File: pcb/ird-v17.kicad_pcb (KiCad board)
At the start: 2 copper layers, 25.4 x 30.5 mm, 21 parts, among them J1 AVR-TPI-6, J2 Conn_02x06_Odd_Even, K1 G6K-2, Q1 NPN 10K, U1 ATtiny20-U, U2 TSOP75438WTT, U3 TLVM365R15RDNR

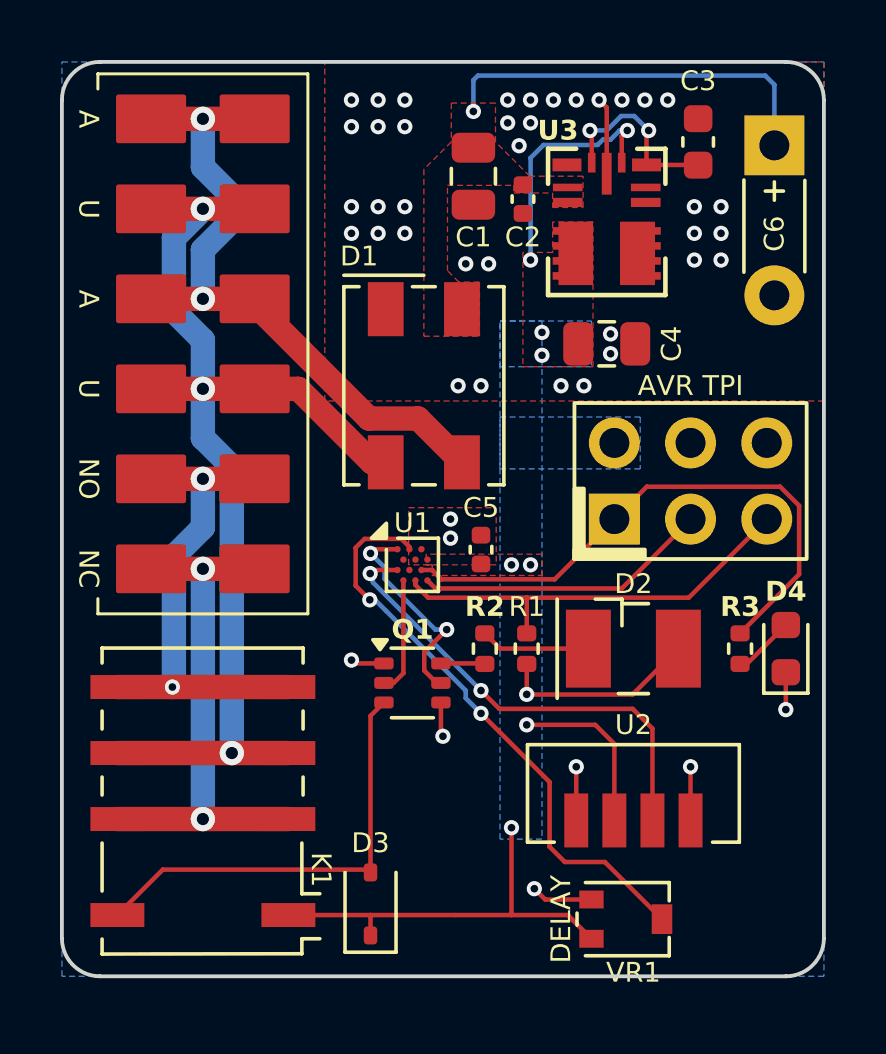
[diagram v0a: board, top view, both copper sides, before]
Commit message: Rearrange pins
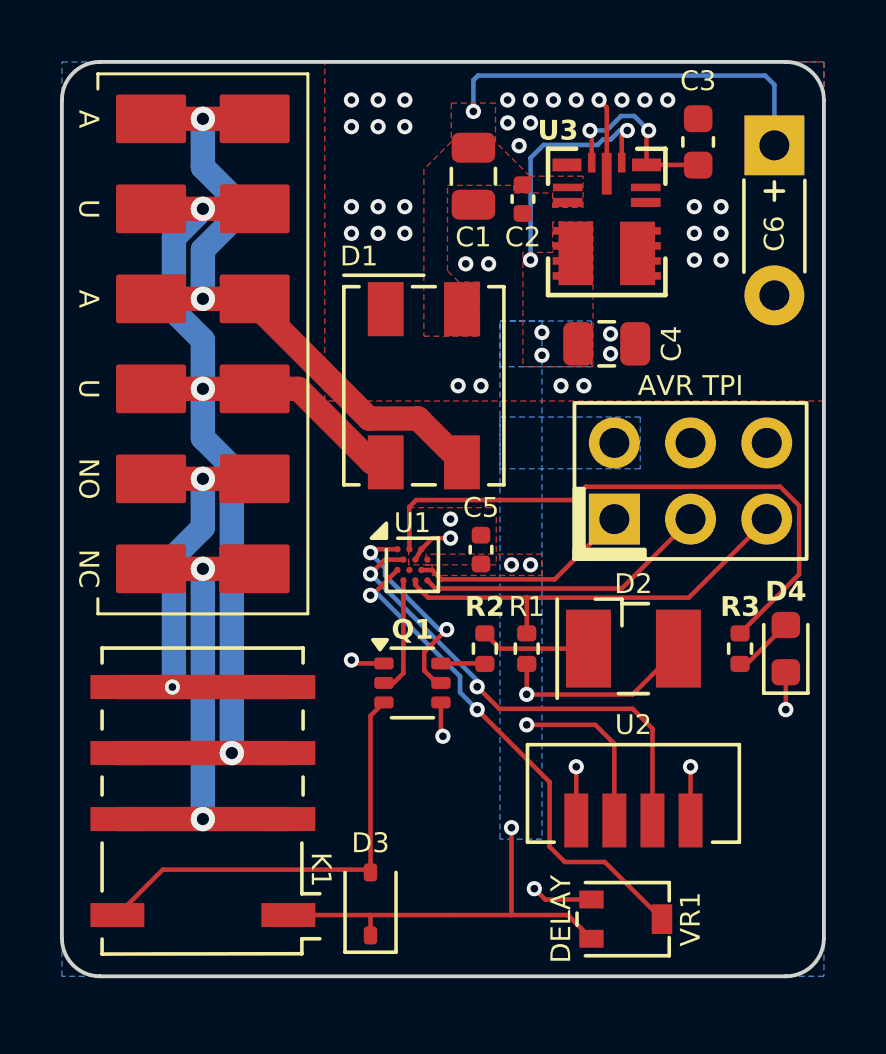
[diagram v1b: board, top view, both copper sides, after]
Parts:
- U2: value TSOP75438WTT -> TSOP75438TT
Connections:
- net OC0A_LED renamed PWMO_LED
- net PA5_RELAY renamed DO_RELAY
- R3 pad 1: TPIDATA -> DO_LED
- U1 pad A3: ADC2_DELAY -> DO_LED
- U1 pad B2: unconnected-(U1-PA6-PadB2) -> DI_SENSE
- U1 pad C1: PA4_SENSE -> AI_DELAY
- U2 pad 3: PA4_SENSE -> DI_SENSE
- VR1 pad 2: ADC2_DELAY -> AI_DELAY
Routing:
- net DO_LED: track 0.00 -> 20.0 mm
- net ADC2_DELAY: track 19.6 -> 0.00 mm, vias 2 -> 0
- net AI_DELAY: track 0.00 -> 17.0 mm, vias 0 -> 2
- net DI_SENSE: track 0.00 -> 16.0 mm, vias 0 -> 2
- net PA4_SENSE: track 15.7 -> 0.00 mm, vias 2 -> 0
- net TPIDATA: track 19.3 -> 7.40 mm
- net GND: track 11.7 -> 13.2 mm
